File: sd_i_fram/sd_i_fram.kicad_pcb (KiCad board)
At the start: 2 copper layers, 39.7 x 42.8 mm, 15 parts, among them J1 Conn_02x05_Odd_Even, J2 Molex 104031

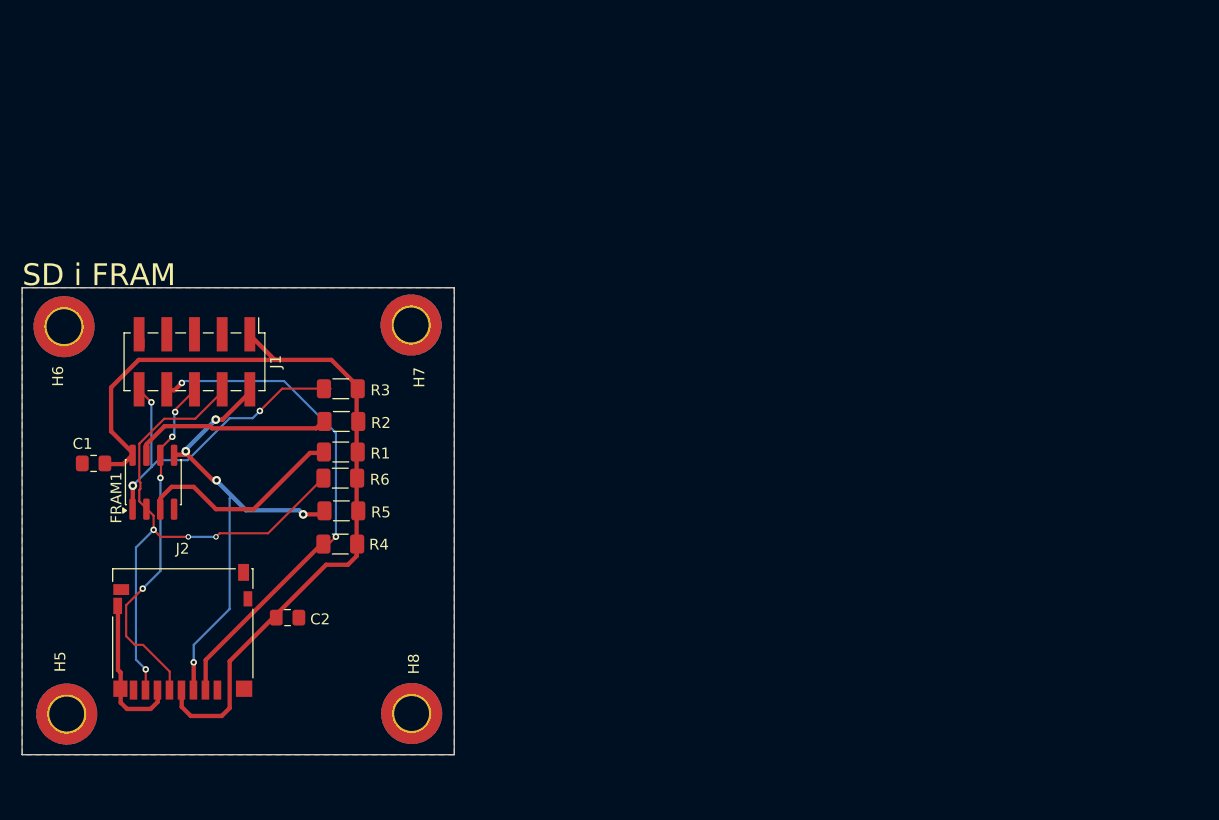
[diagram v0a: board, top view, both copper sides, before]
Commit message: resized. Kanapka
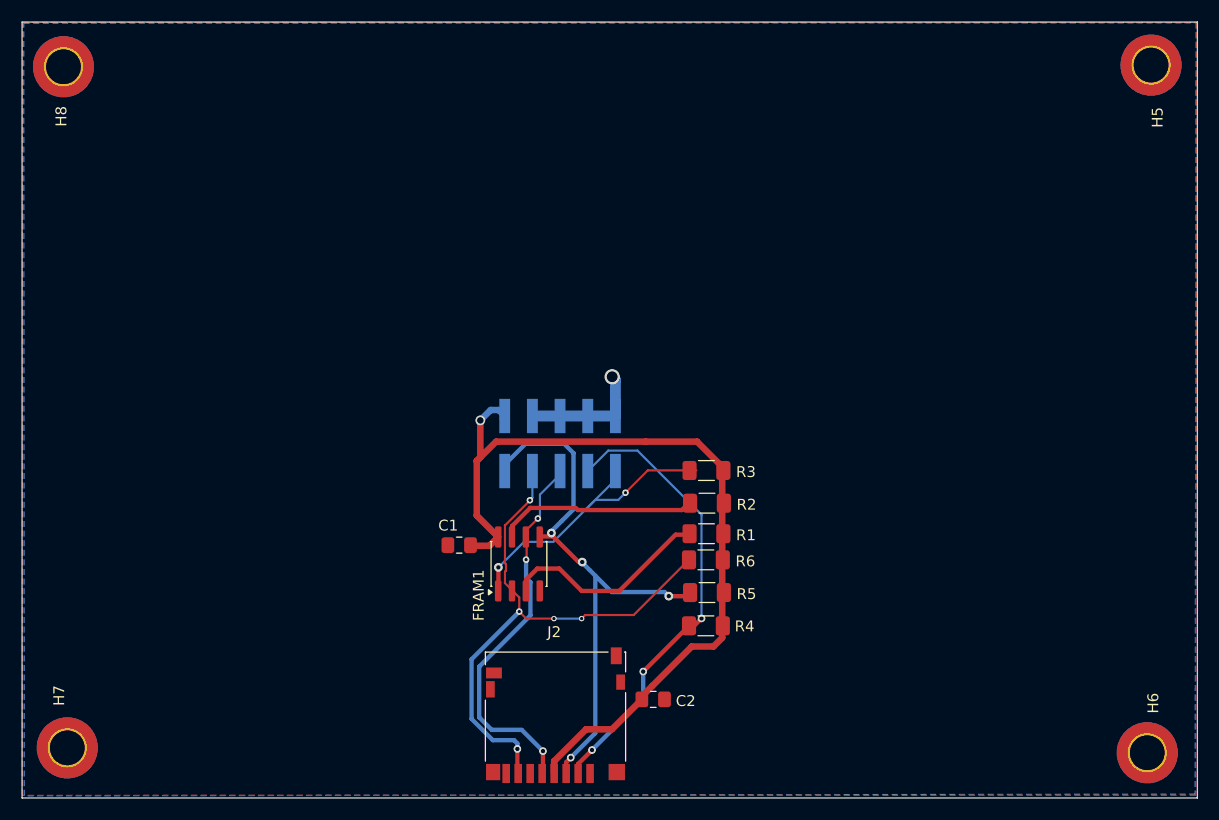
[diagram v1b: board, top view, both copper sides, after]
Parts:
- J1: moved to B.Cu
- moved H5 116.0 mm to (138.7, 3.30), turned to -90 degrees
- moved H6 106.8 mm to (138.3, 66.4), turned to 180 degrees
- moved H8 67.4 mm to (38.9, 3.45), turned to 180 degrees
- moved H7 50.0 mm to (39.2, 66.0), turned to 180 degrees
- moved J2 35.0 mm to (84.0, 63.0)
- moved R2 34.4 mm to (97.9, 43.5)
- moved R5 34.4 mm to (97.9, 51.7)
- moved C2 34.4 mm to (93.0, 61.5)
- moved J1 34.4 mm to (84.4, 38.0)
- moved C1 34.4 mm to (75.2, 47.4)
- moved FRAM1 34.4 mm to (80.6, 49.1)
- moved R1 34.4 mm to (97.8, 46.3)
- moved R3 34.4 mm to (97.8, 40.5)
- moved R4 34.4 mm to (97.8, 54.8)
- moved R6 34.4 mm to (97.8, 48.7)
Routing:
- net /MOSI_2: track 44.7 -> 52.6 mm, vias 5 -> 4
- net /~{SD_CS_2}: track 46.6 -> 42.3 mm, vias 2 -> 3
- net GND_CPU_1: track 14.8 -> 11.3 mm, vias 0 -> 1
- net /SCK_2: track 32.3 -> 35.3 mm, vias 4 -> 3
- net /~{FRAM_CS_2}: track 31.5 -> 28.5 mm, vias 3 -> 2
- net VDD_1: track 80.3 -> 78.7 mm, vias 0 -> 1
- net /MISO_2: track 52.0 -> 52.1 mm, vias 4 -> 5
- added copper zone on B.Cu, net GND_CPU_1
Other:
- board size 39.7 x 42.8 mm -> 107.9 x 71.2 mm
- board text removed: "SD i FRAM"
